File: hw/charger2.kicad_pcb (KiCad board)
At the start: 2 copper layers, 100 x 60 mm, 143 parts, among them J2 Conn_01x08, J3 Conn_01x08, J4 4.5V Power Supply, J5 External ADS1115, J6 Temp, J7 Temp, Q10 AO3400, Q11 AO3400, Q12 AO3400, Q13 AO3400, Q14 AO3400, Q15 AO3400, Q16 AO3400, Q17 AO3400, Q2 AO3400, Q3 AO3400, Q4 AO3400, Q5 AO3400, Q6 AO3400, Q7 AO3400, Q8 AO3400, Q9 AO3400, SW1 Rotary_Encoder_Switch, U1 74HC4050, U10 TP4056, U12 MCP23017_SS, U15 4052, U17 TP4056, U18 TP4056, U19 TP4056, U2 MCP23017_SS, U20 TP4056, U23 ADS1115IDGS, U3 2.2" SPI display, U5 4052, U7 TP4056, U8 TP4056, U9 TP4056

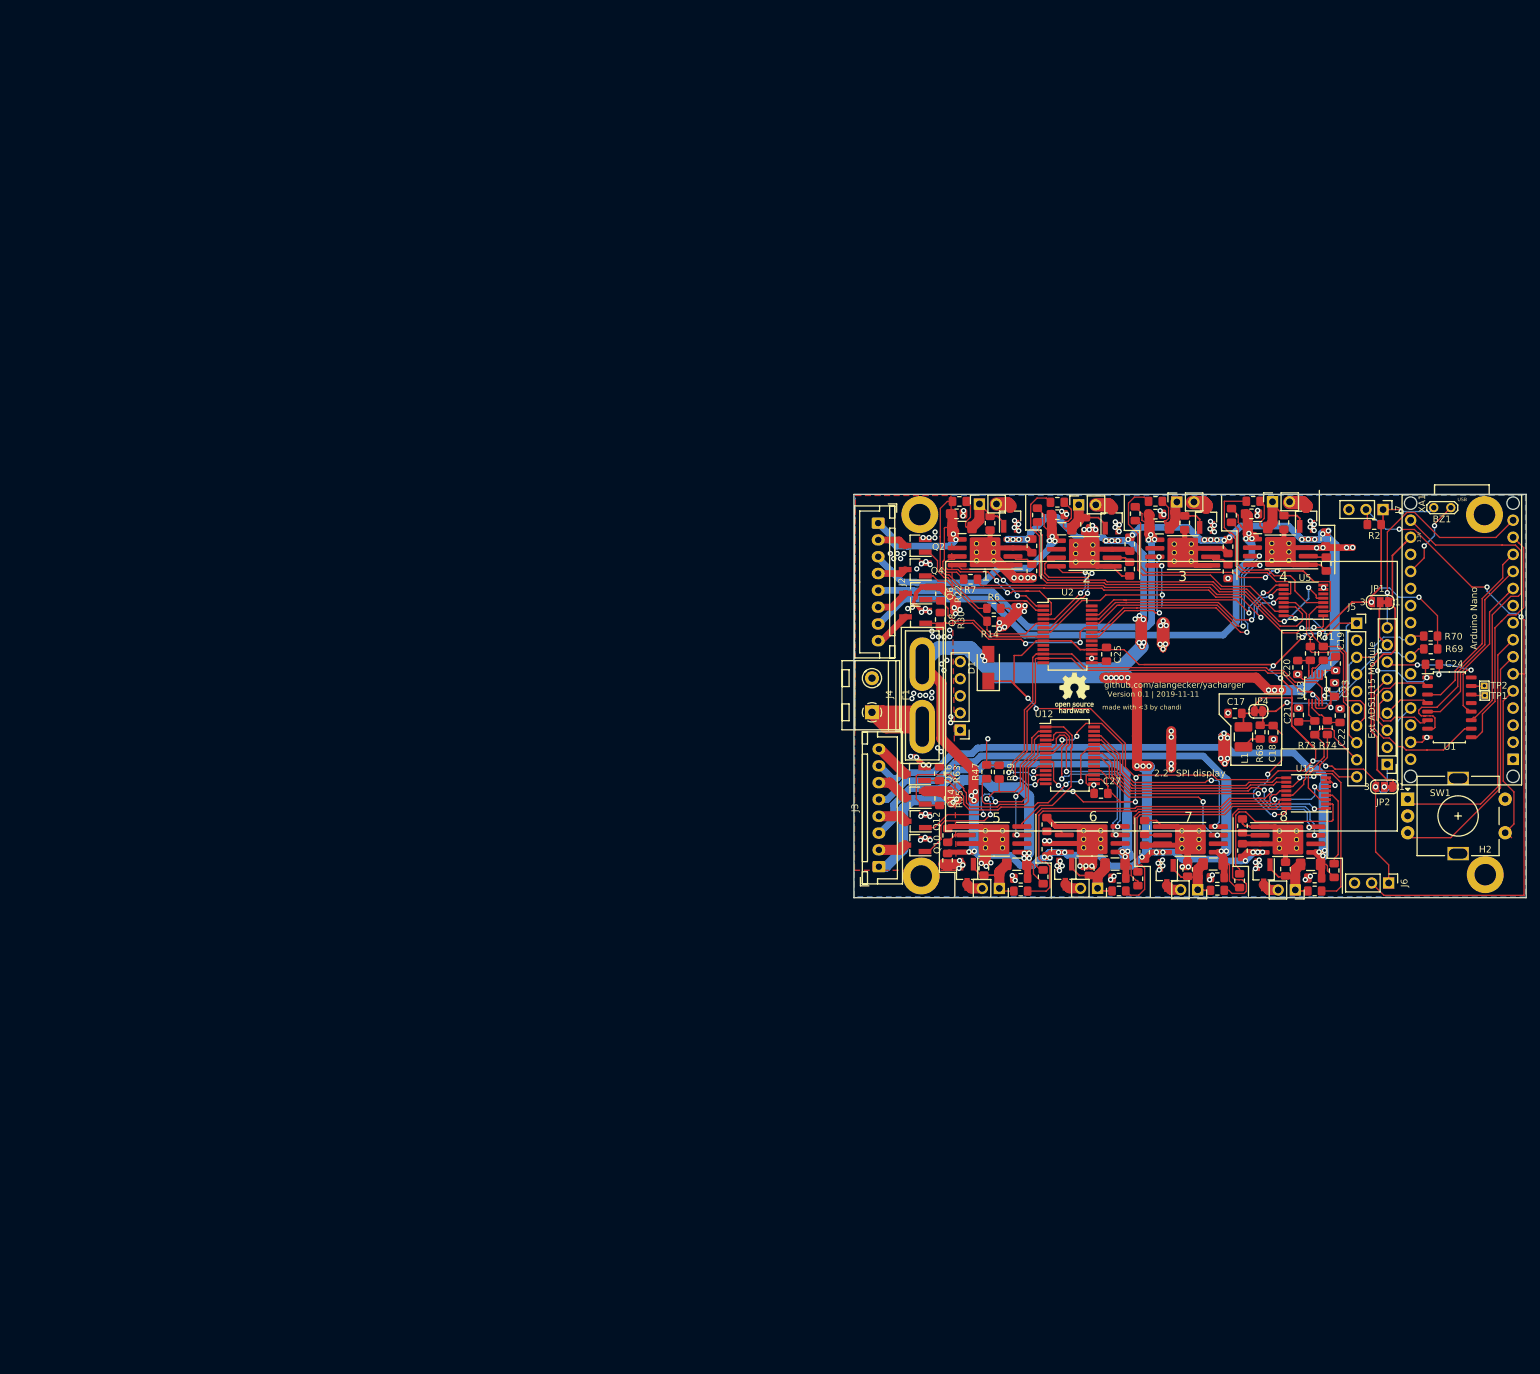
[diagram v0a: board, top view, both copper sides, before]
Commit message: hw: pcb redesign
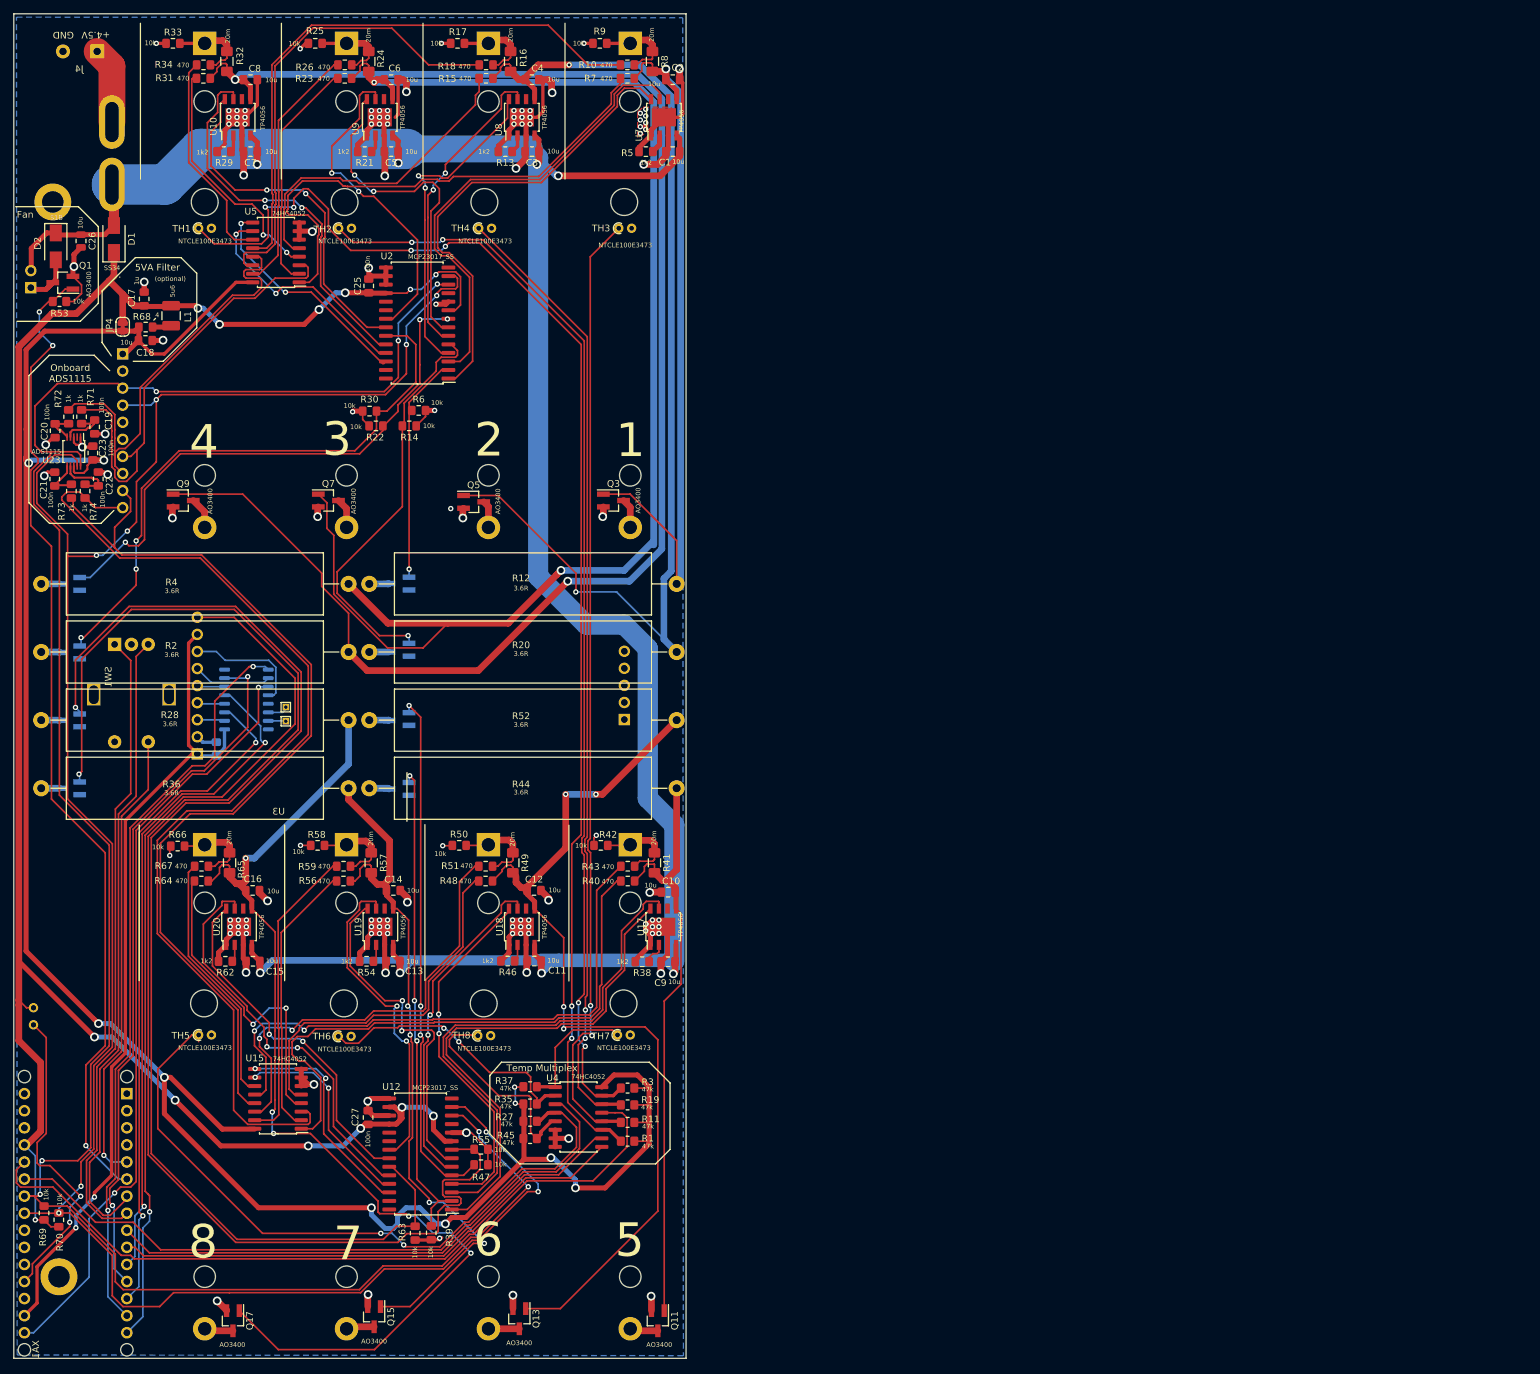
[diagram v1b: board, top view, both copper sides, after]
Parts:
- removed H3, H4: MountingHole, MountingHole:MountingHole_3.2mm_M3_ISO14580_Pad
- removed J2, J3: Conn_01x08, Connector_JST:JST_XH_B8B-XH-A_1x08_P2.50mm_Vertical
- removed J6, J7: Temp, Connector_PinHeader_2.54mm:PinHeader_1x03_P2.54mm_Vertical
- removed JP1: TFT_BL, Jumper:SolderJumper-3_P1.3mm_Bridged12_RoundedPad1.0x1.5mm_NumberLabels
- removed JP2: TFT_VCC, Jumper:SolderJumper-3_P1.3mm_Bridged12_RoundedPad1.0x1.5mm_NumberLabels
- removed the REF** at (145.4, 95.8)
- added C26: 10u, Capacitor_SMD:C_0805_2012Metric, F.Cu at (-2.40, 28.6)
- added D2: S1B, Diode_SMD:D_SMA, F.Cu at (-6.15, 29.4)
- added J1: Fan, Connector_PinSocket_2.54mm:PinSocket_1x02_P2.54mm_Vertical, B.Cu at (-9.86, 35.5)
- added Q1: AO3400, Package_TO_SOT_SMD:SOT-23_Handsoldering, F.Cu at (-5.10, 34.8)
- added R1: 47k, Resistor_SMD:R_0805_2012Metric_Pad1.20x1.40mm_HandSolder, F.Cu at (78.9, 162.5)
- added R11: 47k, Resistor_SMD:R_0805_2012Metric_Pad1.20x1.40mm_HandSolder, F.Cu at (78.9, 159.7)
- added R12: 3.6R, Resistor_THT:R_Axial_Power_L38.0mm_W9.0mm_P45.72mm, F.Cu at (86.2, 79.6)
- added R19: 47k, Resistor_SMD:R_0805_2012Metric_Pad1.20x1.40mm_HandSolder, F.Cu at (78.9, 157.1)
- added R20: 3.6R, Resistor_THT:R_Axial_Power_L38.0mm_W9.0mm_P45.72mm, F.Cu at (86.2, 89.7)
- added R27: 47k, Resistor_SMD:R_0805_2012Metric_Pad1.20x1.40mm_HandSolder, F.Cu at (64.4, 159.5)
- added R28: 3.6R, Resistor_THT:R_Axial_Power_L38.0mm_W9.0mm_P45.72mm, F.Cu at (37.4, 99.9)
- added R3: 47k, Resistor_SMD:R_0805_2012Metric_Pad1.20x1.40mm_HandSolder, F.Cu at (78.9, 154.6)
- added R35: 47k, Resistor_SMD:R_0805_2012Metric_Pad1.20x1.40mm_HandSolder, F.Cu at (64.4, 157.0)
- added R36: 3.6R, Resistor_THT:R_Axial_Power_L38.0mm_W9.0mm_P45.72mm, F.Cu at (37.4, 110.0)
- added R37: 47k, Resistor_SMD:R_0805_2012Metric_Pad1.20x1.40mm_HandSolder, F.Cu at (64.4, 154.4)
- added R4: 3.6R, Resistor_THT:R_Axial_Power_L38.0mm_W9.0mm_P45.72mm, F.Cu at (37.4, 79.6)
- added R44: 3.6R, Resistor_THT:R_Axial_Power_L38.0mm_W9.0mm_P45.72mm, F.Cu at (86.2, 110.0)
- added R45: 47k, Resistor_SMD:R_0805_2012Metric_Pad1.20x1.40mm_HandSolder, F.Cu at (64.4, 162.1)
- added R52: 3.6R, Resistor_THT:R_Axial_Power_L38.0mm_W9.0mm_P45.72mm, F.Cu at (86.2, 99.9)
- added R53: 10k, Resistor_SMD:R_0805_2012Metric_Pad1.20x1.40mm_HandSolder, F.Cu at (-5.60, 37.6)
- added REF**: OSHW-Logo2_7.3x6mm_SilkScreen, Symbol:OSHW-Logo2_7.3x6mm_SilkScreen, B.Cu at (-3.16, 142.6)
- added TH1: NTCLE100E3473, Resistor_THT:R_Axial_DIN0204_L3.6mm_D1.6mm_P1.90mm_Vertical, F.Cu at (15.1, 26.7)
- added TH2: NTCLE100E3473, Resistor_THT:R_Axial_DIN0204_L3.6mm_D1.6mm_P1.90mm_Vertical, F.Cu at (35.9, 26.7)
- added TH3: NTCLE100E3473, Resistor_THT:R_Axial_DIN0204_L3.6mm_D1.6mm_P1.90mm_Vertical, F.Cu at (77.6, 26.7)
- added TH4: NTCLE100E3473, Resistor_THT:R_Axial_DIN0204_L3.6mm_D1.6mm_P1.90mm_Vertical, F.Cu at (56.8, 26.7)
- added TH5: NTCLE100E3473, Resistor_THT:R_Axial_DIN0204_L3.6mm_D1.6mm_P1.90mm_Vertical, F.Cu at (15.1, 146.7)
- added TH6: NTCLE100E3473, Resistor_THT:R_Axial_DIN0204_L3.6mm_D1.6mm_P1.90mm_Vertical, F.Cu at (35.9, 146.9)
- added TH7: NTCLE100E3473, Resistor_THT:R_Axial_DIN0204_L3.6mm_D1.6mm_P1.90mm_Vertical, F.Cu at (77.4, 146.7)
- added TH8: NTCLE100E3473, Resistor_THT:R_Axial_DIN0204_L3.6mm_D1.6mm_P1.90mm_Vertical, F.Cu at (56.6, 146.8)
- added U4: 74HC4052, Package_SO:SO-16_5.3x10.2mm_P1.27mm, F.Cu at (71.6, 158.9)
- BT1, BT2, BT3, BT4, BT5, BT6, BT7, BT8: footprint Connector_PinSocket_2.54mm:PinSocket_1x02_P2.54mm_Vertical -> Battery:BatteryHolder_MPD_BH-18650-PC2; moved to B.Cu
- BZ1, C24, J4, J5, Q10, Q12, Q14, Q16, Q2, Q4, Q6, Q8, U1, U3, XA1: moved to B.Cu
- F1: value Fuse -> 10A; moved to B.Cu
- R2: value 4k7 -> 3.6R; footprint Resistor_SMD:R_0805_2012Metric_Pad1.15x1.40mm_HandSolder -> Resistor_THT:R_Axial_Power_L38.0mm_W9.0mm_P45.72mm
- SW1: value Rotary_Encoder_Switch -> Button; moved to B.Cu
- U10, U17, U18, U19, U20, U7, U8, U9: footprint Package_SO:SOP-8-1EP_4.57x4.57mm_P1.27mm_EP4.57x4.45mm_ThermalVias -> TP4056:TP4056_SOP-8-PP
- U12, U2: footprint Package_SO:SSOP-28_5.3x10.2mm_P0.65mm -> Package_SO:SOIC-28W_7.5x17.9mm_P1.27mm
- U15, U5: value 4052 -> 74HC4052; footprint Package_SO:TSSOP-16_4.4x5mm_P0.65mm -> Package_SO:SO-16_5.3x10.2mm_P1.27mm
- U23: value ADS1115IDGS -> ADS1115
- moved XA1 242.9 mm to (-3.20, 194.8)
- moved R69 222.7 mm to (-7.90, 173.2), turned to 270 degrees
- moved R70 221.8 mm to (-5.70, 174.2), turned to 270 degrees
- moved BZ1 221.2 mm to (-9.47, 142.7), turned to 270 degrees
- moved H2 220.4 mm to (-5.68, 182.7)
- moved H1 218.0 mm to (-6.60, 22.8)
- moved SW1 193.7 mm to (2.60, 88.6), turned to 270 degrees
- moved C21 188.3 mm to (-6.31, 64.0)
- moved R73 188.3 mm to (-3.83, 65.8)
- moved C20 188.1 mm to (-6.25, 56.8)
- moved R74 188.1 mm to (-1.80, 65.8)
- moved C23 188.0 mm to (-0.64, 60.1)
- moved R71 188.0 mm to (-2.32, 54.7)
- moved U23 188.0 mm to (-3.47, 59.9)
- moved C22 188.0 mm to (0.17, 64.0)
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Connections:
- C10 pad 1: /quadcharger2/Battery/L+ -> /quadcharger2/Battery/Bat+'
- C12 pad 1: /quadcharger2/sheet5DC5D930/L+ -> /quadcharger2/sheet5DC5D930/Bat+'
- C14 pad 1: /quadcharger2/sheet5DC5D9EA/L+ -> /quadcharger2/sheet5DC5D9EA/Bat+'
- C16 pad 1: /quadcharger2/sheet5DC5DB5C/L+ -> /quadcharger2/sheet5DC5DB5C/Bat+'
- C2 pad 1: /quadcharger1/Battery/L+ -> /quadcharger1/Battery/Bat+'
- C4 pad 1: /quadcharger1/sheet5DC5D930/L+ -> /quadcharger1/sheet5DC5D930/Bat+'
- C6 pad 1: /quadcharger1/sheet5DC5D9EA/L+ -> /quadcharger1/sheet5DC5D9EA/Bat+'
- C8 pad 1: /quadcharger1/sheet5DC5DB5C/L+ -> /quadcharger1/sheet5DC5DB5C/Bat+'
- Q10 pad 3: /quadcharger2/Battery/L- -> Net-(Q10-Pad3)
- Q11 pad 1: /quadcharger2/Battery/Bat+ -> /quadcharger2/Battery/Bat+'
- Q12 pad 3: /quadcharger2/sheet5DC5D930/L- -> Net-(Q12-Pad3)
- Q13 pad 1: /quadcharger2/sheet5DC5D930/Bat+ -> /quadcharger2/sheet5DC5D930/Bat+'
- Q14 pad 3: /quadcharger2/sheet5DC5D9EA/L- -> Net-(Q14-Pad3)
- Q15 pad 1: /quadcharger2/sheet5DC5D9EA/Bat+ -> /quadcharger2/sheet5DC5D9EA/Bat+'
- Q16 pad 3: /quadcharger2/sheet5DC5DB5C/L- -> Net-(Q16-Pad3)
- Q17 pad 1: /quadcharger2/sheet5DC5DB5C/Bat+ -> /quadcharger2/sheet5DC5DB5C/Bat+'
- Q2 pad 3: /quadcharger1/Battery/L- -> Net-(Q2-Pad3)
- Q3 pad 1: /quadcharger1/Battery/Bat+ -> /quadcharger1/Battery/Bat+'
- Q4 pad 3: /quadcharger1/sheet5DC5D930/L- -> Net-(Q4-Pad3)
- Q5 pad 1: /quadcharger1/sheet5DC5D930/Bat+ -> /quadcharger1/sheet5DC5D930/Bat+'
- Q6 pad 3: /quadcharger1/sheet5DC5D9EA/L- -> Net-(Q6-Pad3)
- Q7 pad 1: /quadcharger1/sheet5DC5D9EA/Bat+ -> /quadcharger1/sheet5DC5D9EA/Bat+'
- Q8 pad 3: /quadcharger1/sheet5DC5DB5C/L- -> Net-(Q8-Pad3)
- Q9 pad 1: /quadcharger1/sheet5DC5DB5C/Bat+ -> /quadcharger1/sheet5DC5DB5C/Bat+'
- R15 pad 1: /quadcharger1/sheet5DC5D930/L+ -> /quadcharger1/sheet5DC5D930/Bat+'
- R16 pad 2: /quadcharger1/sheet5DC5D930/L+ -> /quadcharger1/sheet5DC5D930/Bat+'
- R2 pad 1: +5V -> /quadcharger1/sheet5DC5DB5C/Bat+'
- R2 pad 2: /1wire -> Net-(Q8-Pad3)
- R23 pad 1: /quadcharger1/sheet5DC5D9EA/L+ -> /quadcharger1/sheet5DC5D9EA/Bat+'
- R24 pad 2: /quadcharger1/sheet5DC5D9EA/L+ -> /quadcharger1/sheet5DC5D9EA/Bat+'
- R31 pad 1: /quadcharger1/sheet5DC5DB5C/L+ -> /quadcharger1/sheet5DC5DB5C/Bat+'
- R32 pad 2: /quadcharger1/sheet5DC5DB5C/L+ -> /quadcharger1/sheet5DC5DB5C/Bat+'
- R40 pad 1: /quadcharger2/Battery/L+ -> /quadcharger2/Battery/Bat+'
- R41 pad 2: /quadcharger2/Battery/L+ -> /quadcharger2/Battery/Bat+'
- R48 pad 1: /quadcharger2/sheet5DC5D930/L+ -> /quadcharger2/sheet5DC5D930/Bat+'
- R49 pad 2: /quadcharger2/sheet5DC5D930/L+ -> /quadcharger2/sheet5DC5D930/Bat+'
- R56 pad 1: /quadcharger2/sheet5DC5D9EA/L+ -> /quadcharger2/sheet5DC5D9EA/Bat+'
- R57 pad 2: /quadcharger2/sheet5DC5D9EA/L+ -> /quadcharger2/sheet5DC5D9EA/Bat+'
- R64 pad 1: /quadcharger2/sheet5DC5DB5C/L+ -> /quadcharger2/sheet5DC5DB5C/Bat+'
- R65 pad 2: /quadcharger2/sheet5DC5DB5C/L+ -> /quadcharger2/sheet5DC5DB5C/Bat+'
- R7 pad 1: /quadcharger1/Battery/L+ -> /quadcharger1/Battery/Bat+'
- R8 pad 2: /quadcharger1/Battery/L+ -> /quadcharger1/Battery/Bat+'
- U10 pad 5: /quadcharger1/sheet5DC5DB5C/L+ -> /quadcharger1/sheet5DC5DB5C/Bat+'
- U12 pad 10: Net-(U12-Pad10) -> GND
- U15 pad 6: Net-(U15-Pad6) -> GND
- U17 pad 5: /quadcharger2/Battery/L+ -> /quadcharger2/Battery/Bat+'
- U18 pad 5: /quadcharger2/sheet5DC5D930/L+ -> /quadcharger2/sheet5DC5D930/Bat+'
- U19 pad 5: /quadcharger2/sheet5DC5D9EA/L+ -> /quadcharger2/sheet5DC5D9EA/Bat+'
- U2 pad 10: Net-(U2-Pad10) -> GND
- U20 pad 5: /quadcharger2/sheet5DC5DB5C/L+ -> /quadcharger2/sheet5DC5DB5C/Bat+'
- U3 pad 1: Net-(JP2-Pad2) -> +3V3
- U3 pad 8: Net-(JP1-Pad2) -> +3V3
- U5 pad 6: Net-(U5-Pad6) -> GND
- U7 pad 5: /quadcharger1/Battery/L+ -> /quadcharger1/Battery/Bat+'
- U8 pad 5: /quadcharger1/sheet5DC5D930/L+ -> /quadcharger1/sheet5DC5D930/Bat+'
- U9 pad 5: /quadcharger1/sheet5DC5D9EA/L+ -> /quadcharger1/sheet5DC5D9EA/Bat+'
- XA1 pad D3: /1wire -> /FAN_Control/FAN_PWM
- XA1 pad D6: /MCU/D6 -> /TempMultiplex/S_A
- XA1 pad D7: /MCU/D7 -> /TempMultiplex/S_B
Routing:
- net +5VA: track 70.8 -> 341.2 mm, vias 7 -> 10
- net /MCU/SDA: track 94.3 -> 334.2 mm, vias 3 -> 9
- net /quadcharger1/sheet5DC5DB5C/Bat+': track 0.00 -> 238.9 mm, vias 0 -> 2
- net /quadcharger1/SCK: track 93.3 -> 321.3 mm, vias 4 -> 7
- net /quadcharger1/sheet5DC5D9EA/Bat+': track 0.00 -> 211.1 mm, vias 0 -> 2
- net /TempMultiplex/T4: track 0.00 -> 201.4 mm, vias 0 -> 6
- net /quadcharger2/sheet5DC5D9EA/DE: track 35.6 -> 216.9 mm, vias 0 -> 1
- net /quadcharger1/sheet5DC5D930/Bat+': track 0.00 -> 162.5 mm, vias 0 -> 2
- net /TempMultiplex/T3: track 0.00 -> 162.4 mm, vias 0 -> 4
- net /quadcharger2/sheet5DC5DB5C/Bat+': track 0.00 -> 160.9 mm, vias 0 -> 5
- net /quadcharger2/sheet5DC5DB5C/DE: track 33.8 -> 189.9 mm, vias 2 -> 1
- net /FAN_Control/FAN_PWM: track 0.00 -> 147.5 mm, vias 0 -> 3
- net /TempMultiplex/T2: track 0.00 -> 142.8 mm, vias 0 -> 2
- net /TempMultiplex/T1: track 0.00 -> 142.7 mm, vias 0 -> 2
- net /adc/AIN3: track 19.0 -> 156.8 mm
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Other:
- board size 100 x 60 mm -> 100 x 200 mm
- board text added: "(optional)"
- board text added: "+4.5V"
- board text added: "5VA Filter"
- board text added: "Fan"
- board text added: "GND"
- board text added: "Onboard ADS1115"
- board text added: "Temp Multiplex"
- board text added: "Version 0.2 | 2020-11-28"
- board text removed: "Ext ADS1115 Module"
- board text removed: "Version 0.1 | 2019-11-11"
